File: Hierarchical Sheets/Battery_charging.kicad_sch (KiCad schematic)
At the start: 33 parts, among them J1 USB_C_Receptacle_PowerOnly_6P, U6 ADP1613ARMZ-R7, U8 LM2776

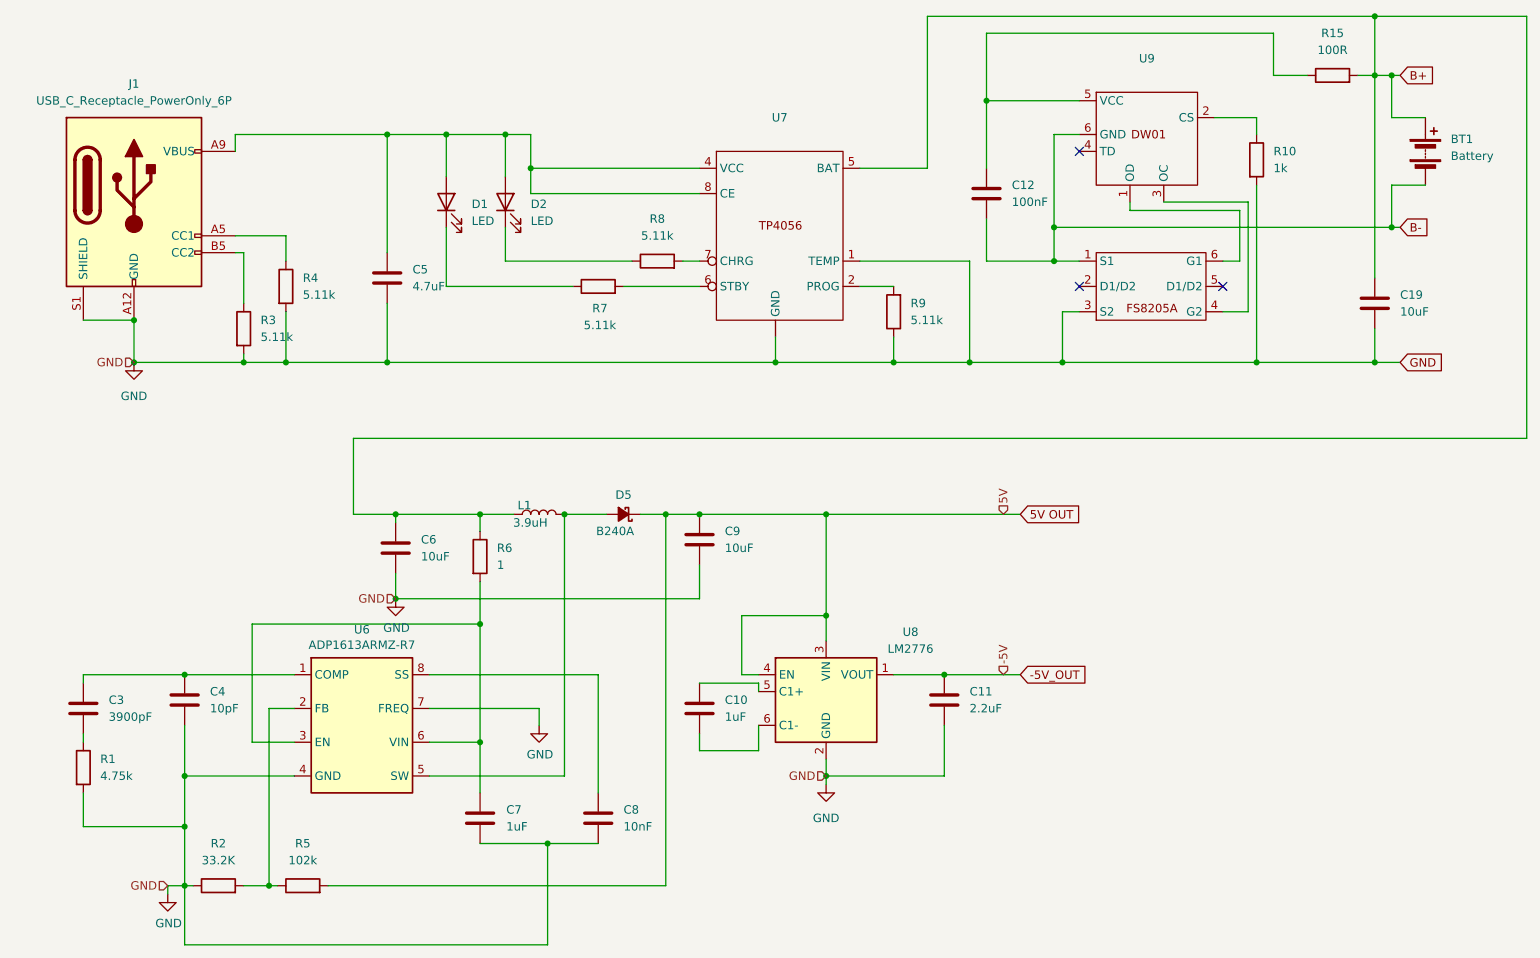
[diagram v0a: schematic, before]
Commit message: Remove extra ref sensor
each module had a reference sensor before, now have single ref sensor comparing to both sensors
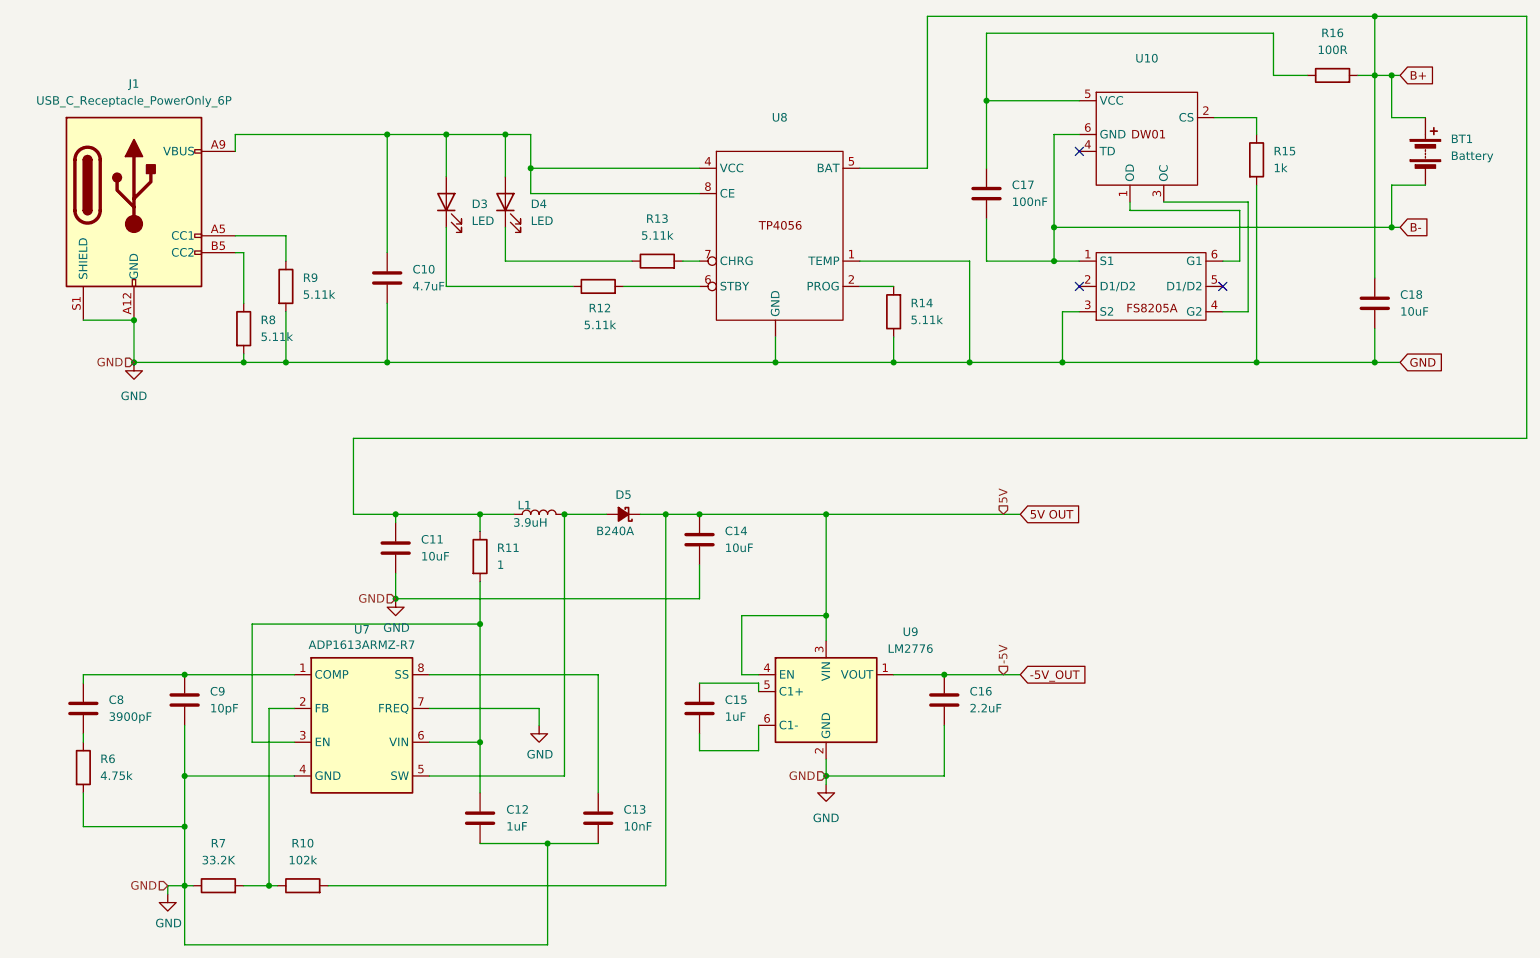
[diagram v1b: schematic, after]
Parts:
- renumbered C5 to C10, C6 to C11, C7 to C12, C8 to C13, C9 to C14, C10 to C15, C11 to C16, C12 to C17, C19 to C18, C3 to C8, C4 to C9, D1 to D3, D2 to D4, R5 to R10, R6 to R11, R7 to R12, R8 to R13, R9 to R14, R10 to R15, R15 to R16, R1 to R6, R2 to R7, R3 to R8, R4 to R9, U9 to U10, U10 to U11, U6 to U7, U7 to U8, U8 to U9

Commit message: Revert "Remove extra ref sensor"
This reverts commit 7f0b0207ac24b991faee57c630f393e10dd69dda.
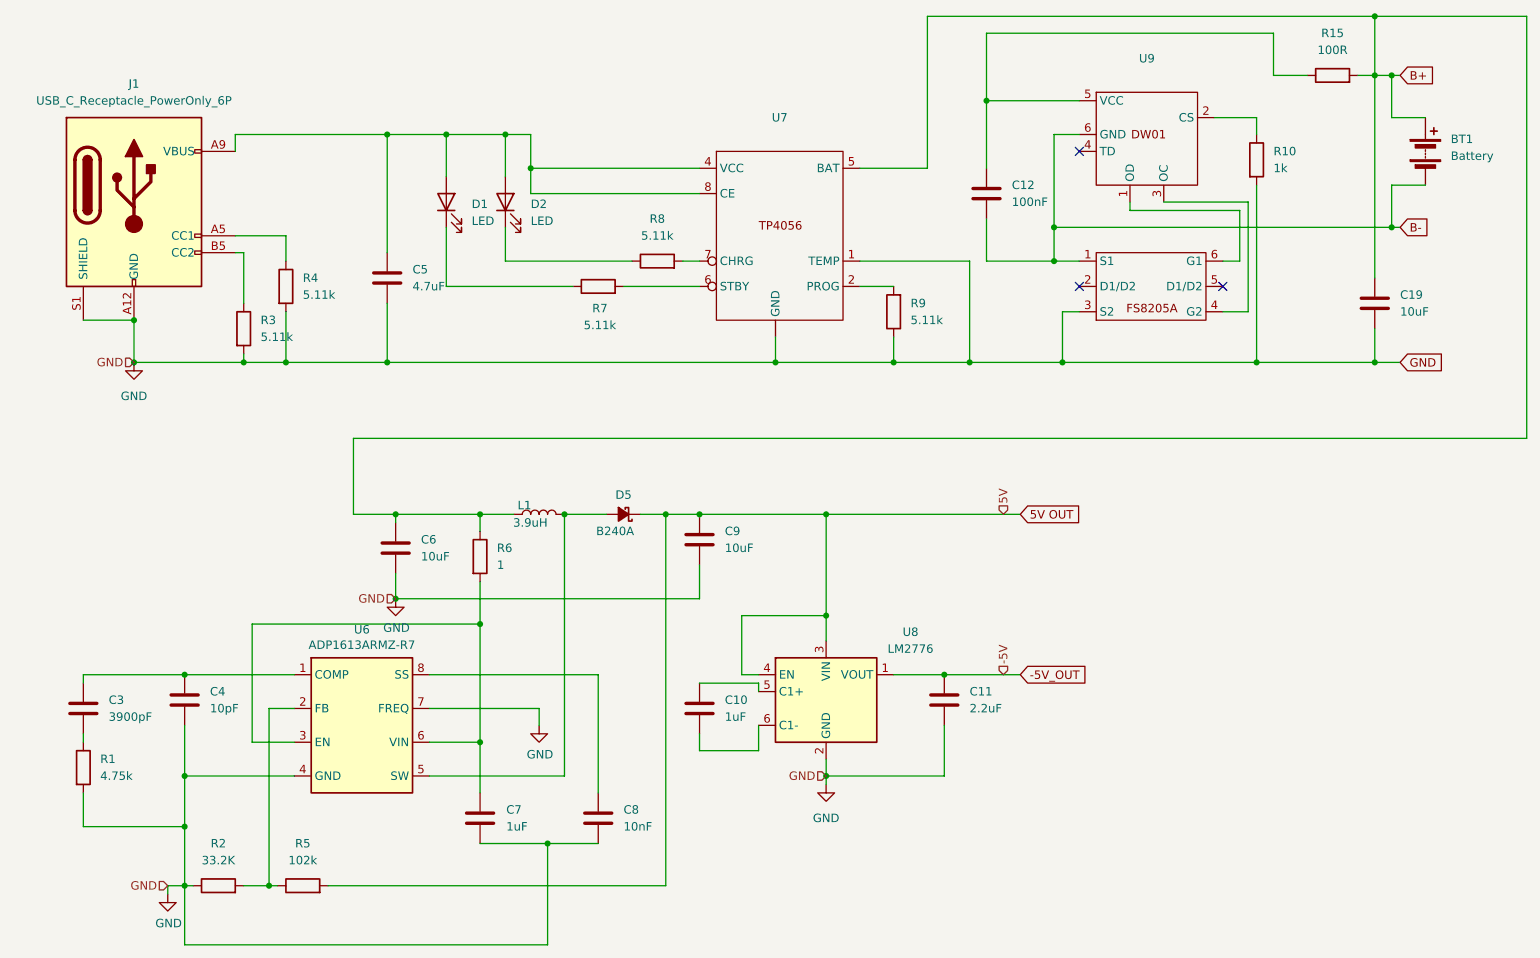
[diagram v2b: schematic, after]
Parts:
- renumbered C15 to C10, C16 to C11, C17 to C12, C18 to C19, C8 to C3, C9 to C4, C10 to C5, C11 to C6, C12 to C7, C13 to C8, C14 to C9, D3 to D1, D4 to D2, R6 to R1, R15 to R10, R16 to R15, R7 to R2, R8 to R3, R9 to R4, R10 to R5, R11 to R6, R12 to R7, R13 to R8, R14 to R9, U11 to U10, U7 to U6, U8 to U7, U9 to U8, U10 to U9
